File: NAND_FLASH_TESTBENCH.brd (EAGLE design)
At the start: 32.2 x 24.9 mm, 25 parts, among them IC1 S35ML04G300WHI000

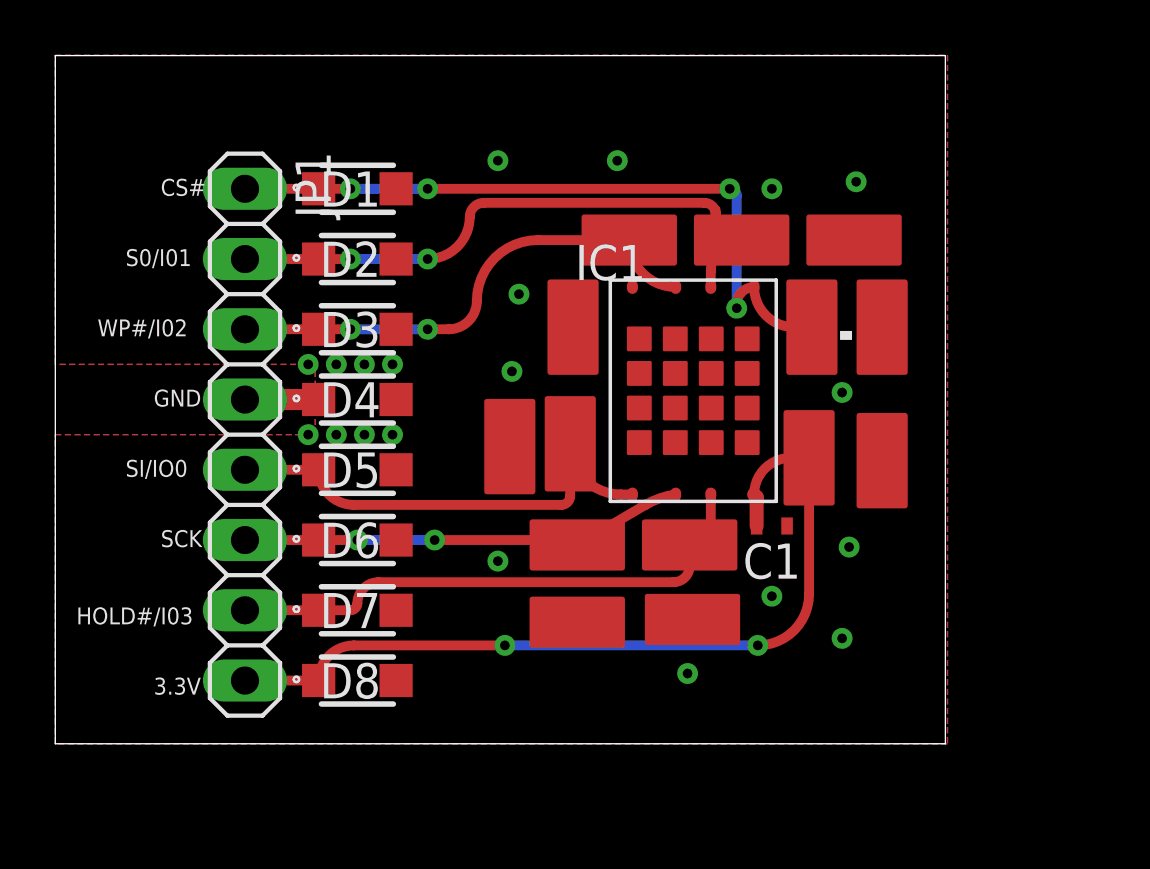
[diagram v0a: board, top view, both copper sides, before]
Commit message: board rev_1
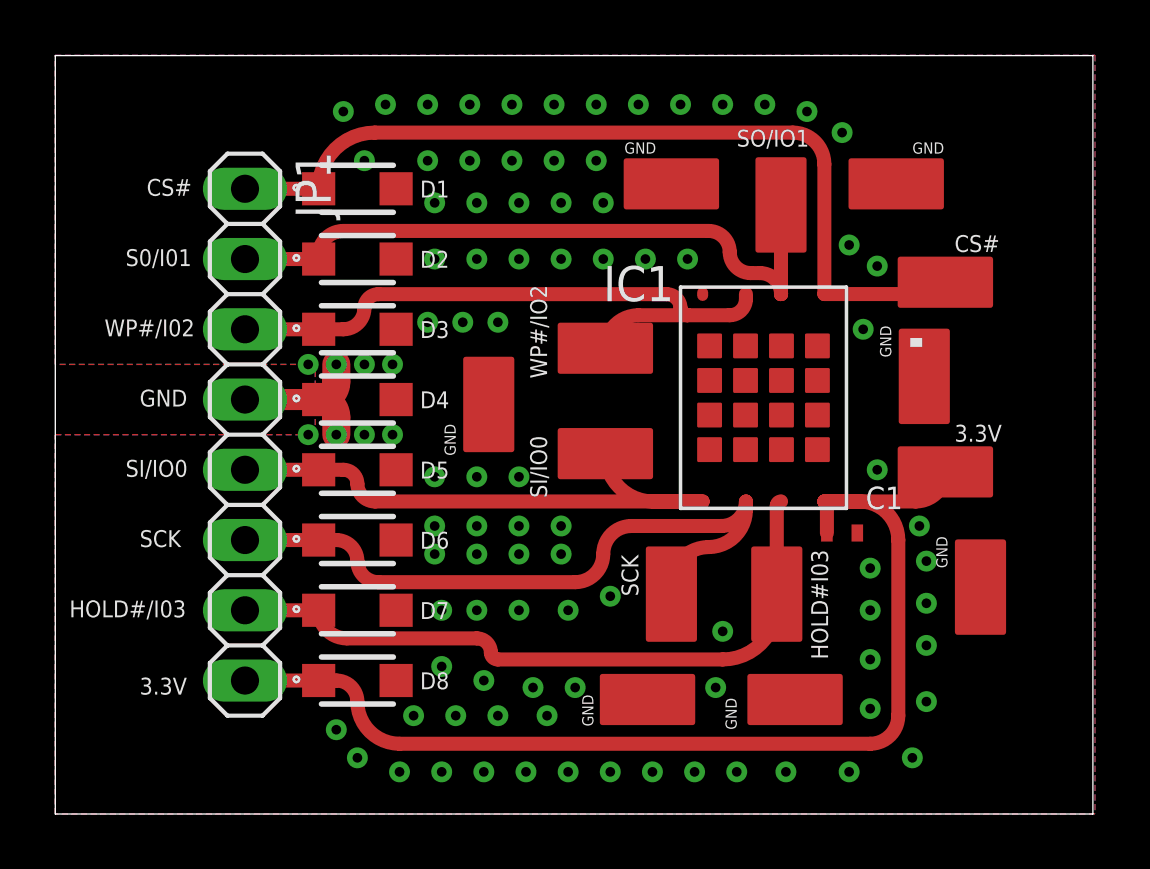
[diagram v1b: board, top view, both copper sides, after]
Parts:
- moved TP12 7.18 mm to (54.6, 25.1), turned to 90 degrees
- moved TP11 5.79 mm to (58.7, 30.0)
- moved TP1 4.19 mm to (56.6, 38.4), turned to 270 degrees
- moved TP2 4.10 mm to (53.3, 40.4), turned to 0 degrees
- moved TP13 3.78 mm to (49.3, 25.1)
- moved TP10 3.78 mm to (46.7, 41.9), turned to 270 degrees
- moved TP3 3.25 mm to (47.8, 37.8), turned to 90 degrees
- moved TP5 3.06 mm to (47.8, 34.0), turned to 90 degrees
- moved C1 2.55 mm to (54.6, 30.2)
- moved IC1 2.55 mm to (48.8, 39.1)
- moved TP4 2.54 mm to (54.9, 41.9)
- moved TP9 2.34 mm to (56.6, 37.6)
- moved TP8 2.30 mm to (56.6, 31.5), turned to 270 degrees
- moved TP14 1.70 mm to (40.9, 36.6)
- moved TP6 1.27 mm to (47.5, 29.7), turned to 180 degrees
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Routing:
- net 3.3V: track 30.4 -> 40.7 mm, vias 2 -> 0
- net SCK: track 16.1 -> 24.4 mm, vias 2 -> 0
- net CS#: track 25.7 -> 31.5 mm, vias 4 -> 0
- net WP#/IO2: track 17.6 -> 22.8 mm, vias 2 -> 0
- net HOLD#/IO3: track 19.6 -> 24.6 mm
- net SI/IO0: track 17.3 -> 21.3 mm
- net GND: track 2.66 -> 5.73 mm, vias 20 -> 95
- net SO/IO1: track 22.9 -> 24.1 mm, vias 2 -> 0
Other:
- board size 32.2 x 24.9 mm -> 37.5 x 27.4 mm
- board text added: "BAJA SAE ELECTRICAL NAND FLASH TESTBENCH DESIGNED BY RYAN THAI 2021-2022 Part S35ML04G300WHI000"
- board text added: "HOLD#I03"
- board text added: "SO/IO1"
- board text added: "WP#/IO2"
- board text removed: "BAJA SAE ELECTRICAL NAND FLASH TESTBENCH DESIGNED BY RYAN THAI"
